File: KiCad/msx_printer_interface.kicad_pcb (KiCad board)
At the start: 2 copper layers, 65.7 x 53 mm, 11 parts, among them J1 MSX Cartridge Connector, J2 Conn_02x07_Top_Bottom, U1 ATF22V10C-15PU, U2 74HC273

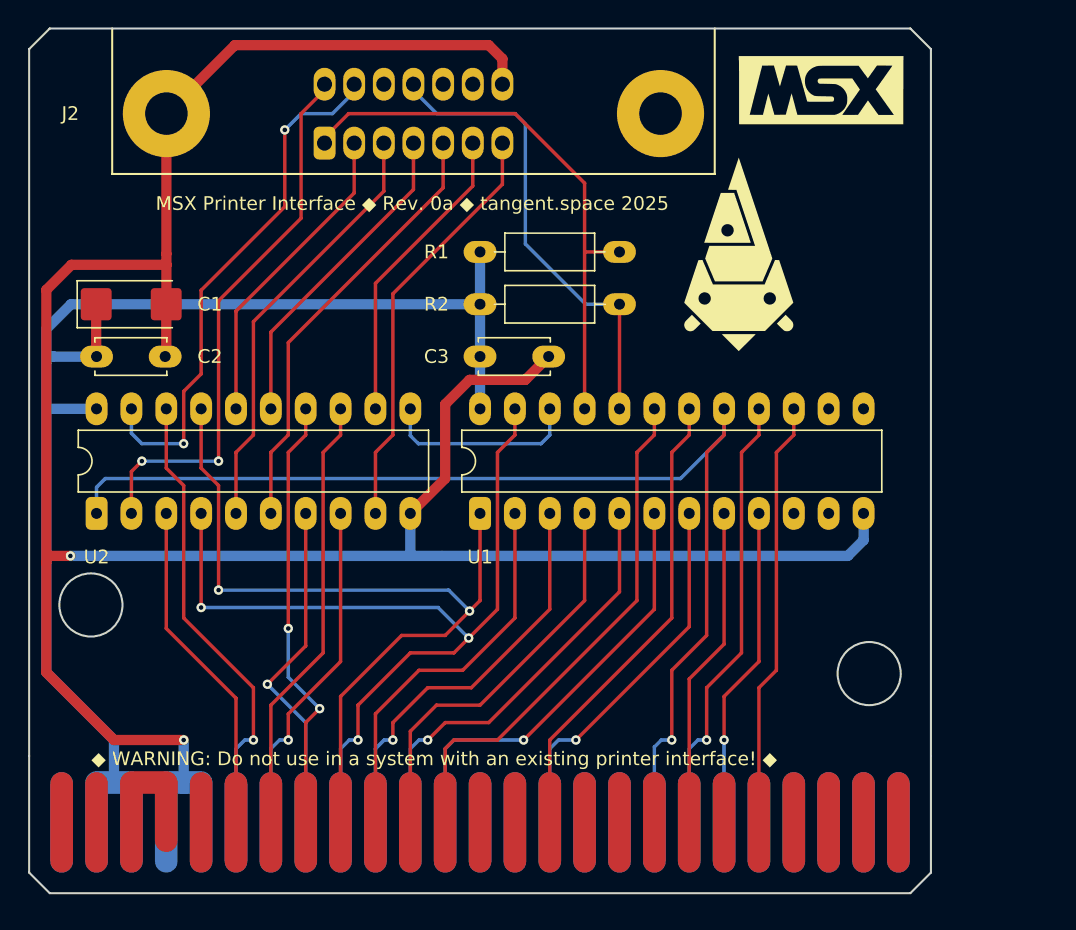
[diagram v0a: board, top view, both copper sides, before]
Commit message: Update msx_printer_interface.kicad_pcb
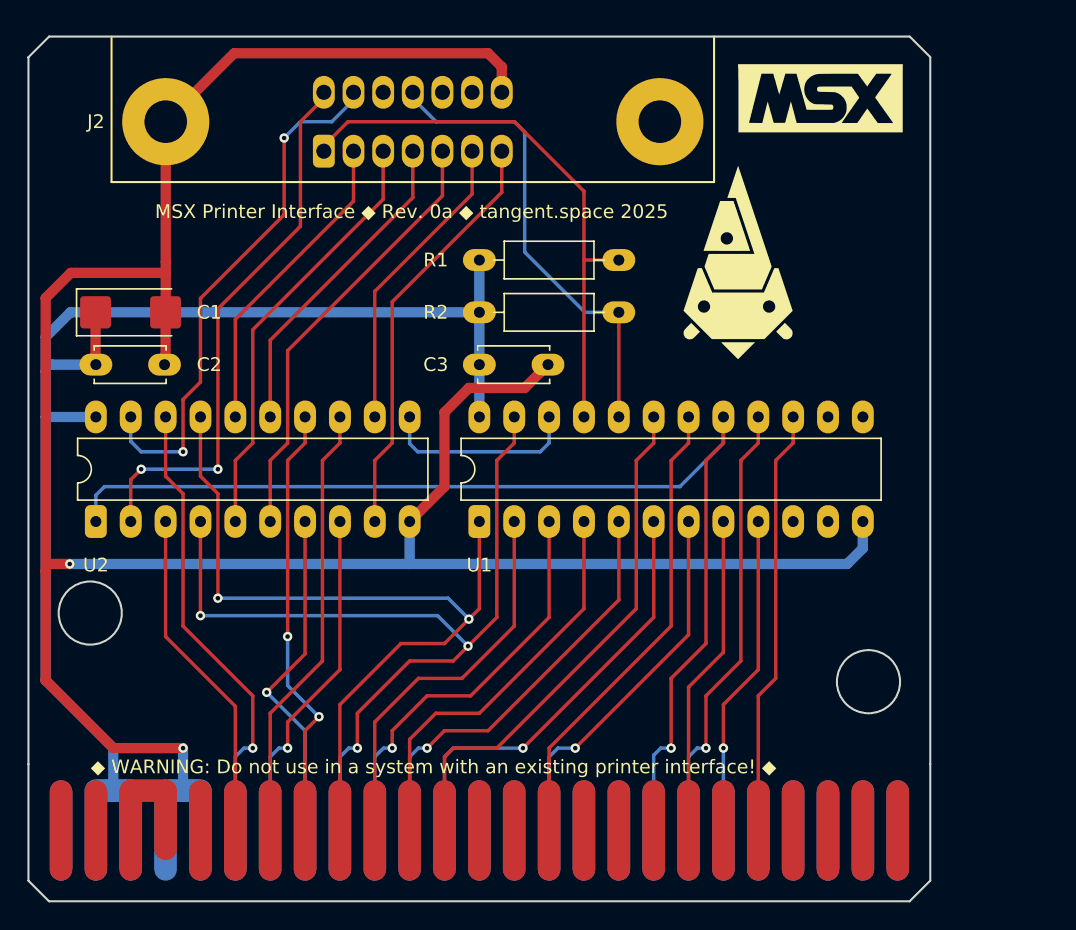
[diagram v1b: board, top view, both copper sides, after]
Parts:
- moved C1 0.59 mm to (36.4, 35.6)
- moved R2 0.59 mm to (72.0, 35.6)
- moved G*** 0.59 mm to (86.7, 20.0)
- moved G*** 0.59 mm to (80.7, 31.9)
- moved J2 0.59 mm to (35.0, 11.0)
- moved J1 0.59 mm to (2.50, 11.0)
- moved R1 0.59 mm to (72.0, 31.8)
- moved C2 0.59 mm to (33.9, 39.4)
- moved U2 0.59 mm to (33.9, 50.8)
- moved C3 0.59 mm to (61.9, 39.4)
- moved U1 0.59 mm to (61.9, 50.8)
